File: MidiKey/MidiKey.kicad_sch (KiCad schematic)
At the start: 17 parts, among them J1 Conn_01x07, SW1 SW_Push, SW2 SW_Push, SW3 SW_Push, SW4 RotaryEncoder_Switch_MP, U1 XIAO-ESP32-S3

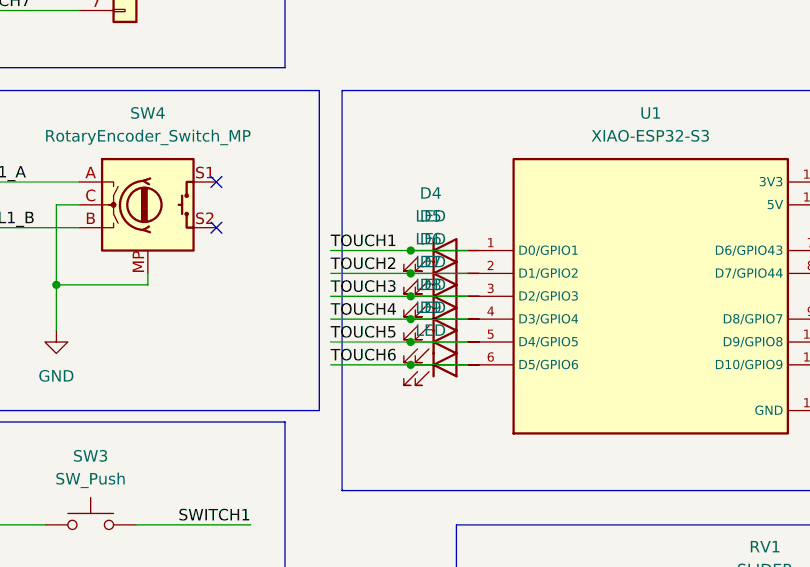
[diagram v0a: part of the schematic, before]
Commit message: Add files via upload
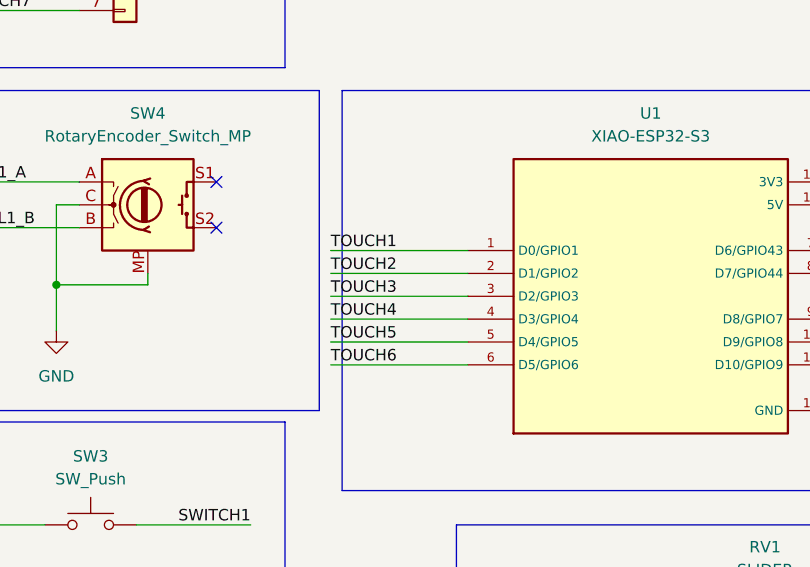
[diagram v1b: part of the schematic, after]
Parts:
- removed D4, D5, D6, D7, D8, D9: LED, symbol Device:LED
